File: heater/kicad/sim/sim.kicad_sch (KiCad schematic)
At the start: 4 parts, among them U1 ${SIM.PARAMS}

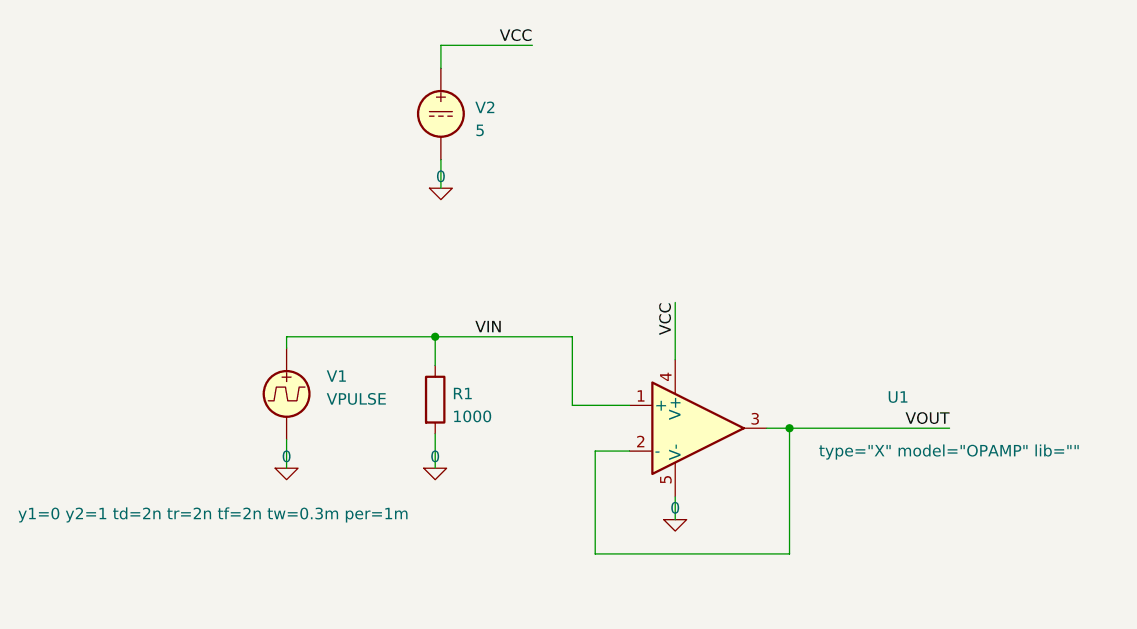
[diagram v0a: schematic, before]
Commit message: Work in spice sim.
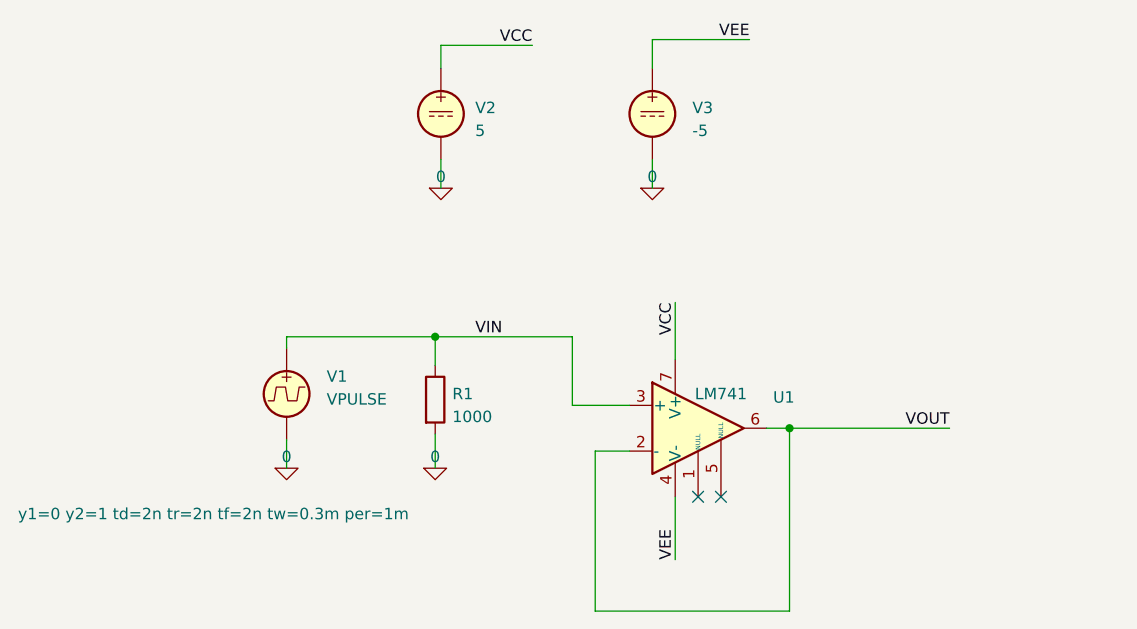
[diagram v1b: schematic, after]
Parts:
- removed U1: ${SIM.PARAMS}, symbol Simulation_SPICE:OPAMP
- added U1: LM741, symbol Amplifier_Operational:LM741
- added V3: -5, symbol Simulation_SPICE:VDC
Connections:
- net 0: now also V3.2
- net VCC: now also U1.7 (V+)
- net VIN: now also U1.3 (+)
- net VOUT: now also U1.2 (-), U1.6
- new net VEE: U1.4 (V-), V3.1
- no-connect marks 0 -> 2
